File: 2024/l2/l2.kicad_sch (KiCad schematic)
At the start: 13 parts, among them J1 Conn_01x04, J2 Conn_01x02, J3 Conn_01x04, Q1 IRF540N, U1 DEV-15583, U2 VNH5019A-E

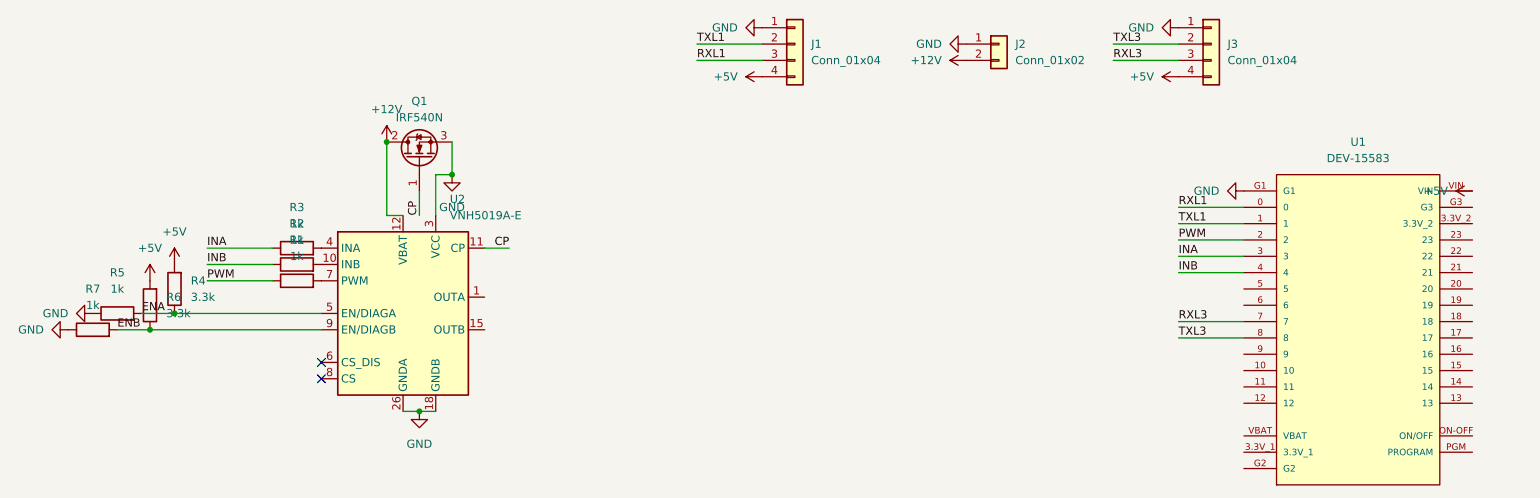
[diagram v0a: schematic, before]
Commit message: 31/7 final
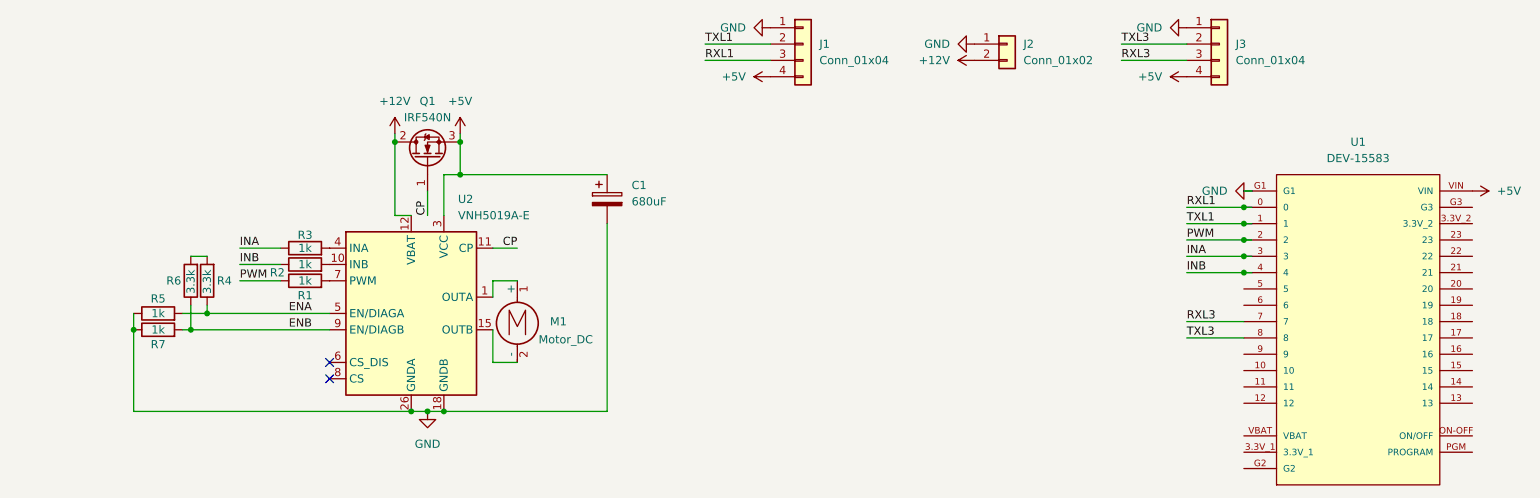
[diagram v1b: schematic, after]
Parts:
- added C1: 680uF, symbol Device:C_Polarized
- added M1: Motor_DC, symbol Motor:Motor_DC
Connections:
- net +5V: now also Q1.3 (S), U2.13 (VCC), U2.23 (VCC), U2.3 (VCC), U2.31 (VCC), C1.1; no longer R4.2, R6.2
- net GND: now also C1.2; no longer Q1.3 (S), U2.13 (VCC), U2.23 (VCC), U2.3 (VCC), U2.31 (VCC)
- net at U2.1 (OUTA), U2.25 (OUTA), U2.30 (OUTA)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: now also M1.1 (+)
- net at U2.15 (OUTB), U2.16 (OUTB), U2.21 (OUTB)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: now also M1.2 (-)
- new net: R4.2, R6.2
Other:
- moved on the sheet: J1, J2, J3, Q1, R1, R2, R3, R4, R5, R6, R7, U2
